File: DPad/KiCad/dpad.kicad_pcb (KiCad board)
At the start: 2 copper layers, 49 x 36 mm, 13 parts, among them M3 MountingHole_3.2mm_M3, SW1 SW_Push, SW2 SW_Push, SW3 SW_Push, SW4 SW_Push

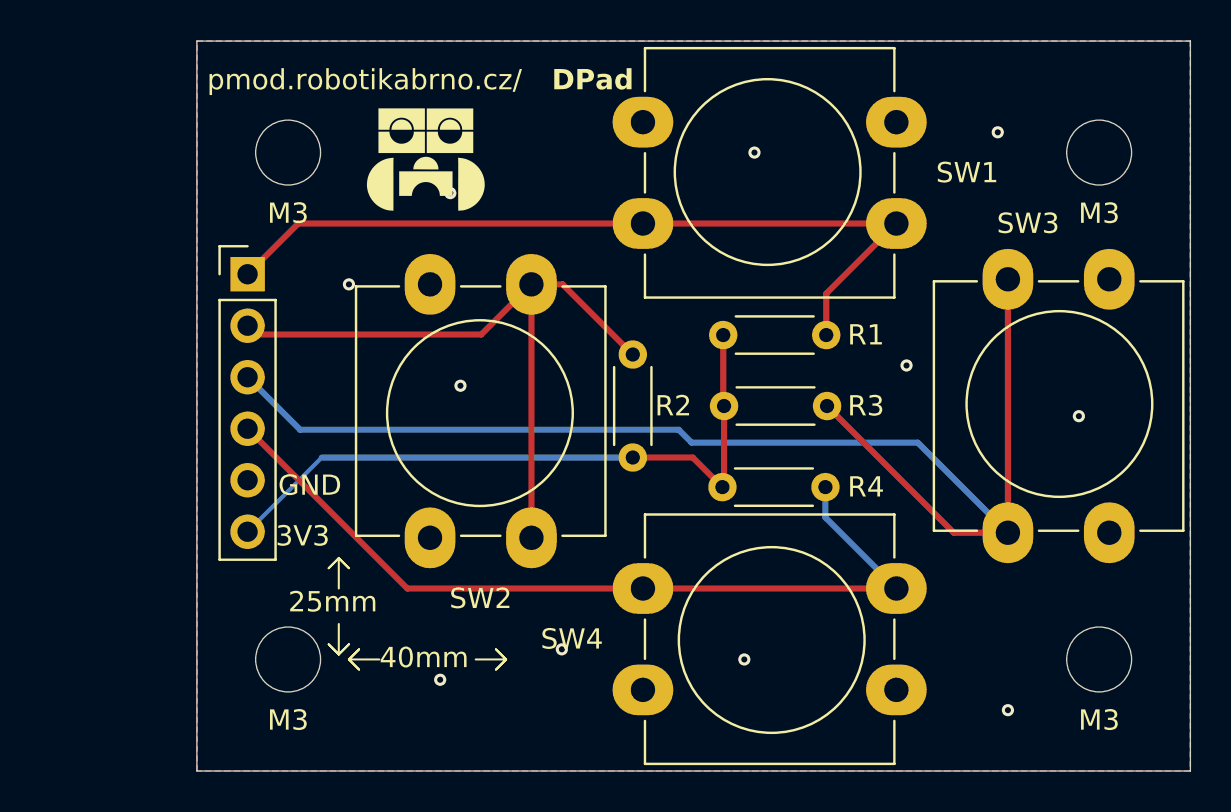
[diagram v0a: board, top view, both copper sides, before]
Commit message: Deployed 7db42b7 with MkDocs version: 1.6.0
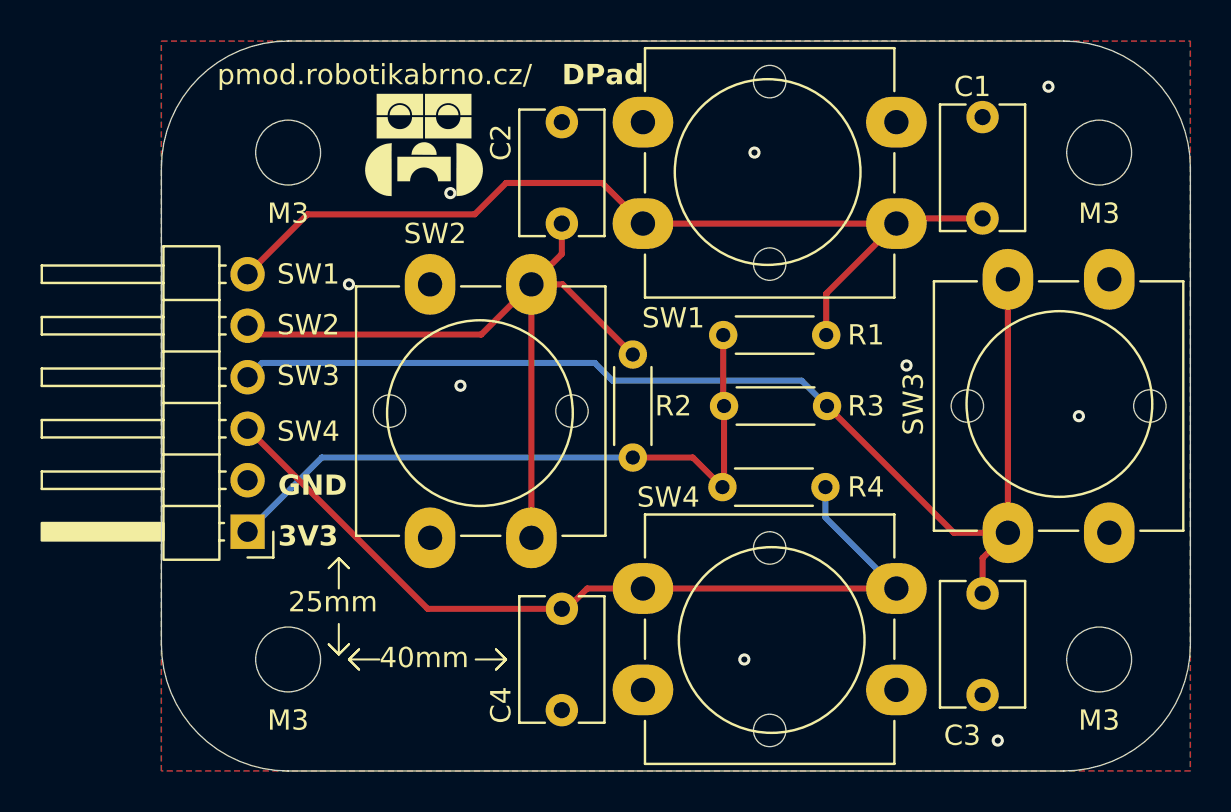
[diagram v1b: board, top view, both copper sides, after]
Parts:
- added C1: 1uF, Custom:C_Disc_D6.0mm_W4mm_P5.00mm, F.Cu at (127.2, 90.8)
- added C2: 1uF, Custom:C_Disc_D6.0mm_W4mm_P5.00mm, F.Cu at (106.5, 91.0)
- added C3: 1uF, Custom:C_Disc_D6.0mm_W4mm_P5.00mm, F.Cu at (127.2, 119.2)
- added C4: 1uF, Custom:C_Disc_D6.0mm_W4mm_P5.00mm, F.Cu at (106.5, 120.0)
- PMOD1: footprint Connector_PinHeader_2.54mm:PinHeader_1x06_P2.54mm_Vertical -> Connector_PinHeader_2.54mm:PinHeader_1x06_P2.54mm_Horizontal
- SW1, SW2, SW3, SW4: footprint Button_Switch_THT:SW_PUSH-12mm_Wuerth-430476085716 -> Custom:SW_PUSH-12mm
- moved PMOD1 8.77 mm to (82.2, 98.5)
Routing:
- net IO3: track 64.7 -> 57.3 mm
- net IO1: track 40.0 -> 46.0 mm
- net IO2: track 34.1 -> 37.8 mm
- net IO4: track 41.7 -> 42.5 mm
- net /GND: vias 11 -> 9
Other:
- board size 49 x 36 mm -> 50.8 x 36 mm
- board text added: "SW2"
- board text added: "SW3"
- board text added: "SW4"
